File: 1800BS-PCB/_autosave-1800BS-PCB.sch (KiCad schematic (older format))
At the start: 24 parts, among them SW1 SW_Push, U1 ATmega32U4-AU, Y1 16MHz

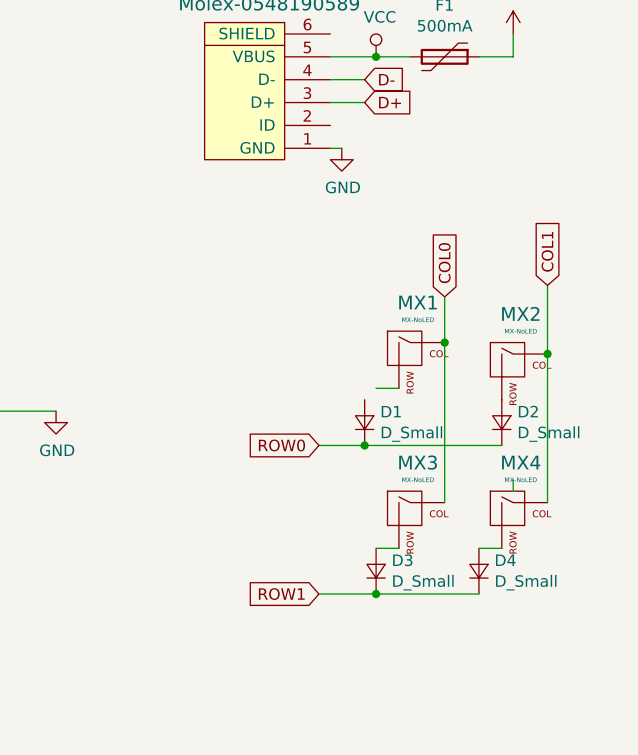
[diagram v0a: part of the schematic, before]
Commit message: PCB Routed
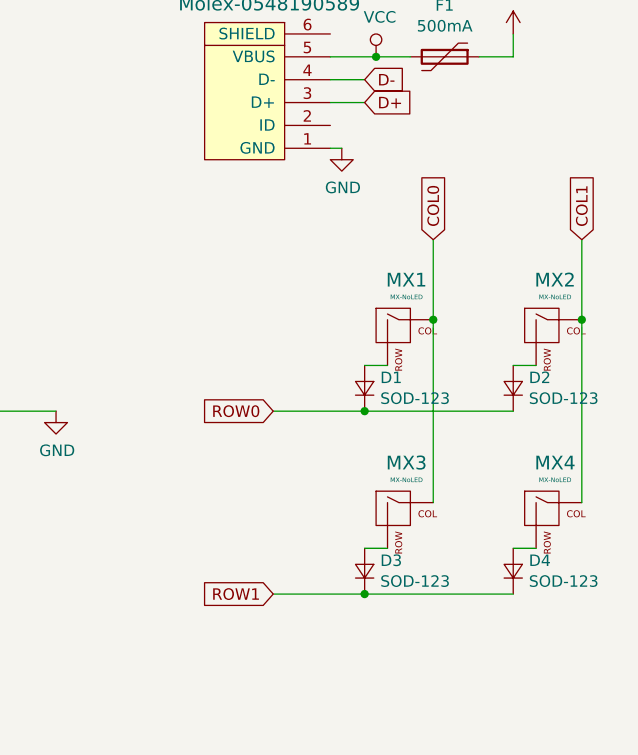
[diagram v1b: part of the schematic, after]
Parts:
- D1, D2, D3, D4: value D_Small -> SOD-123
- MX1, MX2, MX3, MX4: footprint MX_Alps_Hybrid:MX-10U-NoLED -> MX_Alps_Hybrid:MX-1U-NoLED
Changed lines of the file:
@@
 $Comp
 L MX_Alps_Hybrid:MX-NoLED MX1
-U 1 1 5EB7D32A
-P 8250 4100
-F 0 "MX1" H 8283 4323 60  0000 C CNN
-F 1 "MX-NoLED" H 8283 4249 20  0000 C CNN
-F 2 "MX_Alps_Hybrid:MX-10U-NoLED" H 7625 4075 60  0001 C CNN
-F 3 "" H 7625 4075 60  0001 C CNN
-	1    8250 4100
+U 1 1 5EBC80F8
+P 8200 4000
+F 0 "MX1" H 8233 4223 60  0000 C CNN
+F 1 "MX-NoLED" H 8233 4149 20  0000 C CNN
+F 2 "MX_Alps_Hybrid:MX-1U-NoLED" H 7575 3975 60  0001 C CNN
+F 3 "" H 7575 3975 60  0001 C CNN
+	1    8200 4000
 	1    0    0    -1
 $EndComp
+Wire Wire Line
+	8150 4150 8050 4150
 $Comp
 L Device:D_Small D1
-U 1 1 5EB800B1
-P 8050 4400
-F 0 "D1" V 8096 4332 50  0000 R CNN
-F 1 "D_Small" V 8005 4332 50  0000 R CNN
-F 2 "Diode_SMD:D_SOD-123" V 8050 4400 50  0001 C CNN
-F 3 "~" V 8050 4400 50  0001 C CNN
-	1    8050 4400
+U 1 1 5EBCC199
+P 8050 4250
+F 0 "D1" V 8096 4182 50  0000 R CNN
+F 1 "SOD-123" V 8005 4182 50  0000 R CNN
+F 2 "Diode_SMD:D_SOD-123" V 8050 4250 50  0001 C CNN
+F 3 "~" V 8050 4250 50  0001 C CNN
+	1    8050 4250
+	0    -1   -1   0
+$EndComp
+$Comp
+L MX_Alps_Hybrid:MX-NoLED MX2
+U 1 1 5EBCD95F
+P 8850 4000
+F 0 "MX2" H 8883 4223 60  0000 C CNN
+F 1 "MX-NoLED" H 8883 4149 20  0000 C CNN
+F 2 "MX_Alps_Hybrid:MX-1U-NoLED" H 8225 3975 60  0001 C CNN
+F 3 "" H 8225 3975 60  0001 C CNN
+	1    8850 4000
+	1    0    0    -1
+$EndComp
+Wire Wire Line
+	8800 4150 8700 4150
+$Comp
+L Device:D_Small D2
+U 1 1 5EBCD966
+P 8700 4250
+F 0 "D2" V 8746 4182 50  0000 R CNN
+F 1 "SOD-123" V 8655 4182 50  0000 R CNN
+F 2 "Diode_SMD:D_SOD-123" V 8700 4250 50  0001 C CNN
+F 3 "~" V 8700 4250 50  0001 C CNN
+	1    8700 4250
+	0    -1   -1   0
+$EndComp
+$Comp
+L MX_Alps_Hybrid:MX-NoLED MX3
+U 1 1 5EBD0AA3
+P 8200 4800
+F 0 "MX3" H 8233 5023 60  0000 C CNN
+F 1 "MX-NoLED" H 8233 4949 20  0000 C CNN
+F 2 "MX_Alps_Hybrid:MX-1U-NoLED" H 7575 4775 60  0001 C CNN
+F 3 "" H 7575 4775 60  0001 C CNN
+	1    8200 4800
+	1    0    0    -1
+$EndComp
+Wire Wire Line
+	8150 4950 8050 4950
+$Comp
+L Device:D_Small D3
+U 1 1 5EBD0AAA
+P 8050 5050
+F 0 "D3" V 8096 4982 50  0000 R CNN
+F 1 "SOD-123" V 8005 4982 50  0000 R CNN
+F 2 "Diode_SMD:D_SOD-123" V 8050 5050 50  0001 C CNN
+F 3 "~" V 8050 5050 50  0001 C CNN
+	1    8050 5050
+	0    -1   -1   0
+$EndComp
+$Comp
+L MX_Alps_Hybrid:MX-NoLED MX4
+U 1 1 5EBD2CE2
+P 8850 4800
+F 0 "MX4" H 8883 5023 60  0000 C CNN
+F 1 "MX-NoLED" H 8883 4949 20  0000 C CNN
+F 2 "MX_Alps_Hybrid:MX-1U-NoLED" H 8225 4775 60  0001 C CNN
+F 3 "" H 8225 4775 60  0001 C CNN
+	1    8850 4800
+	1    0    0    -1
+$EndComp
+Wire Wire Line
+	8800 4950 8700 4950
+$Comp
+L Device:D_Small D4
+U 1 1 5EBD2CE9
+P 8700 5050
+F 0 "D4" V 8746 4982 50  0000 R CNN
+F 1 "SOD-123" V 8655 4982 50  0000 R CNN
+F 2 "Diode_SMD:D_SOD-123" V 8700 5050 50  0001 C CNN
+F 3 "~" V 8700 5050 50  0001 C CNN
+	1    8700 5050
 	0    -1   -1   0
 $EndComp
 Wire Wire Line
-	8200 4250 8100 4250
-$Comp
-L MX_Alps_Hybrid:MX-NoLED MX2
-U 1 1 5EB82FD6
-P 8700 4150
-F 0 "MX2" H 8733 4373 60  0000 C CNN
-F 1 "MX-NoLED" H 8733 4299 20  0000 C CNN
-F 2 "MX_Alps_Hybrid:MX-10U-NoLED" H 8075 4125 60  0001 C CNN
-F 3 "" H 8075 4125 60  0001 C CNN
-	1    8700 4150
-	1    0    0    -1
-$EndComp
-$Comp
-L MX_Alps_Hybrid:MX-NoLED MX3
-U 1 1 5EB859DD
-P 8250 4800
-F 0 "MX3" H 8283 5023 60  0000 C CNN
-F 1 "MX-NoLED" H 8283 4949 20  0000 C CNN
-F 2 "MX_Alps_Hybrid:MX-10U-NoLED" H 7625 4775 60  0001 C CNN
-F 3 "" H 7625 4775 60  0001 C CNN
-	1    8250 4800
-	1    0    0    -1
-$EndComp
-$Comp
-L Device:D_Small D3
-U 1 1 5EB859E3
-P 8100 5050
-F 0 "D3" V 8146 4982 50  0000 R CNN
-F 1 "D_Small" V 8055 4982 50  0000 R CNN
-F 2 "Diode_SMD:D_SOD-123" V 8100 5050 50  0001 C CNN
-F 3 "~" V 8100 5050 50  0001 C CNN
-	1    8100 5050
-	0    -1   -1   0
-$EndComp
+	9000 4750 9000 3950
+Connection ~ 9000 3950
 Wire Wire Line
-	8200 4950 8100 4950
-$Comp
-L MX_Alps_Hybrid:MX-NoLED MX4
-U 1 1 5EB86E42
-P 8700 4800
-F 0 "MX4" H 8733 5023 60  0000 C CNN
-F 1 "MX-NoLED" H 8733 4949 20  0000 C CNN
-F 2 "MX_Alps_Hybrid:MX-10U-NoLED" H 8075 4775 60  0001 C CNN
-F 3 "" H 8075 4775 60  0001 C CNN
-	1    8700 4800
-	1    0    0    -1
-$EndComp
-$Comp
-L Device:D_Small D4
-U 1 1 5EB86E48
-P 8550 5050
-F 0 "D4" V 8596 4982 50  0000 R CNN
-F 1 "D_Small" V 8505 4982 50  0000 R CNN
-F 2 "Diode_SMD:D_SOD-123" V 8550 5050 50  0001 C CNN
-F 3 "~" V 8550 5050 50  0001 C CNN
-	1    8550 5050
-	0    -1   -1   0
-$EndComp
+	9000 3950 9000 3600
 Wire Wire Line
-	8650 4950 8550 4950
+	8350 4750 8350 3950
+Connection ~ 8350 3950
 Wire Wire Line
-	8700 4700 8700 4650
+	8350 3950 8350 3600
 Wire Wire Line
-	8850 4100 8850 3800
+	8700 4350 8050 4350
+Connection ~ 8050 4350
 Wire Wire Line
-	8550 5150 8100 5150
-Connection ~ 8100 5150
+	8050 4350 7650 4350
 Wire Wire Line
-	8100 5150 7850 5150
-$Comp
-L Device:D_Small D2
-U 1 1 5EB9C0C6
-P 8650 4400
-F 0 "D2" V 8696 4332 50  0000 R CNN
-F 1 "D_Small" V 8605 4332 50  0000 R CNN
-F 2 "Diode_SMD:D_SOD-123" V 8650 4400 50  0001 C CNN
-F 3 "~" V 8650 4400 50  0001 C CNN
-	1    8650 4400
-	0    -1   -1   0
-$EndComp
+	8700 5150 8050 5150
+Connection ~ 8050 5150
 Wire Wire Line
-	8850 4750 8850 4100
-Connection ~ 8850 4100
-Wire Wire Line
-	8400 3850 8400 4050
-Connection ~ 8400 4050
-Wire Wire Line
-	8400 4050 8400 4750
-Wire Wire Line
-	8650 4500 8050 4500
-Connection ~ 8050 4500
-Wire Wire Line
-	8050 4500 7850 4500
-Text GLabel 8400 3850 1    50   Input ~ 0
+	8050 5150 7650 5150
+Text GLabel 8350 3600 1    50   Input ~ 0
 COL0
-Text GLabel 8850 3800 1    50   Input ~ 0
+Text GLabel 9000 3600 1    50   Input ~ 0
 COL1
-Text GLabel 7850 4500 0    50   Input ~ 0
+Text GLabel 7650 4350 0    50   Input ~ 0
 ROW0
-Text GLabel 7850 5150 0    50   Input ~ 0
+Text GLabel 7650 5150 0    50   Input ~ 0
 ROW1
 $EndSCHEMATC

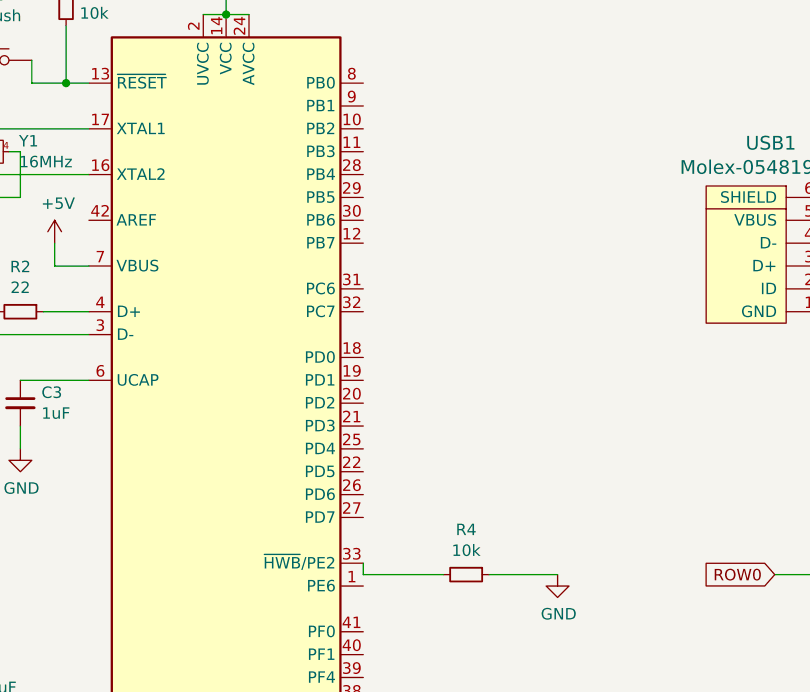
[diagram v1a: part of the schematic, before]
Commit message: Rough draft pcb
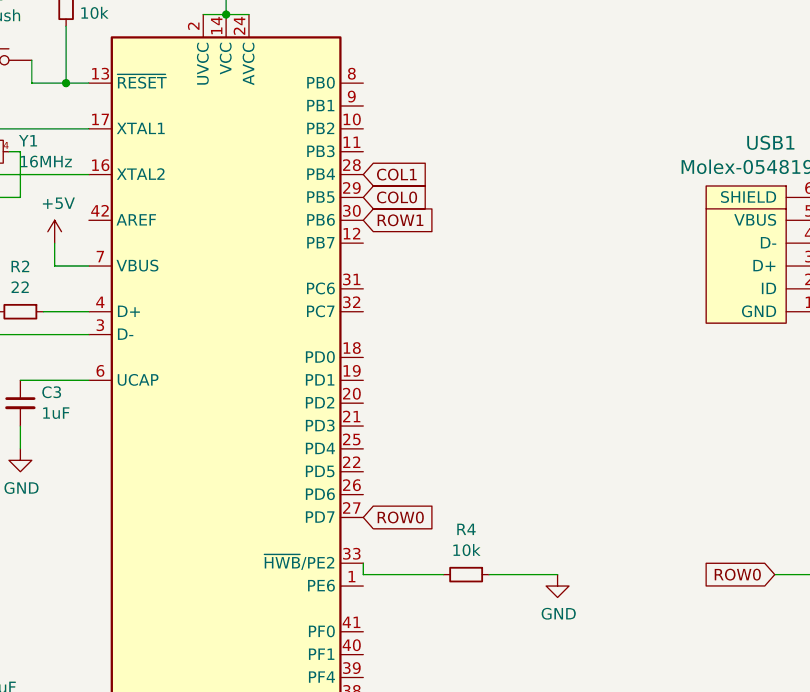
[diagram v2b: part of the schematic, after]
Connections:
- net COL0: now also U1.29 (PB5)
- net COL1: now also U1.28 (PB4)
- net ROW0: now also U1.27 (PD7)
- net ROW1: now also U1.30 (PB6)
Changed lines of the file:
@@
 Text GLabel 7650 5150 0    50   Input ~ 0
 ROW1
+Text GLabel 5850 2600 2    50   Input ~ 0
+COL1
+Text GLabel 5850 2700 2    50   Input ~ 0
+COL0
+Text GLabel 5850 2800 2    50   Input ~ 0
+ROW1
+Text GLabel 5850 4100 2    50   Input ~ 0
+ROW0
 $EndSCHEMATC
